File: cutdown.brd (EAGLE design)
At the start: 94 x 100.3 mm, 133 parts, among them J1 RBF_PLUG, Q1 IPB120P04P4L03ATMA1, Q2 SBC817-40LT1G, Q3 SBC817-40LT1G, SW1 M2012LL2W30, U1 ATSAMD21G-A, U2 ATTINY85V-10S, U3 MPL3115A2, U4 R-783.3-0.5_DC-DC, U5 R-783.3-0.5_DC-DC, U6 CD4013B, U7 MC14106BDR2G, X1 ZX62D-B-5PA8, X2 BU-SMA-V, X3 JST-XH-02-PIN-LONG-PAD, X4 JST-XH-02-PIN-LONG-PAD

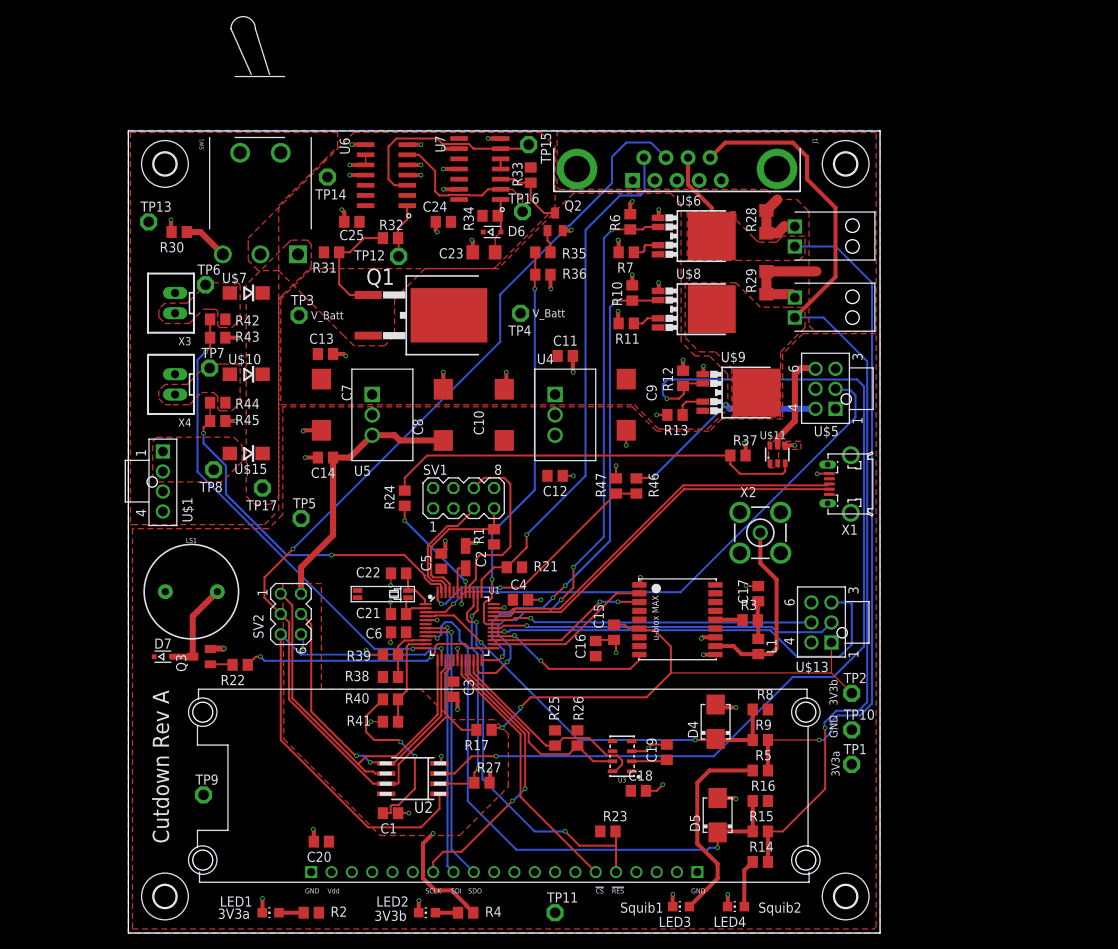
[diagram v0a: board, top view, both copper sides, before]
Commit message: Rev B Hardware
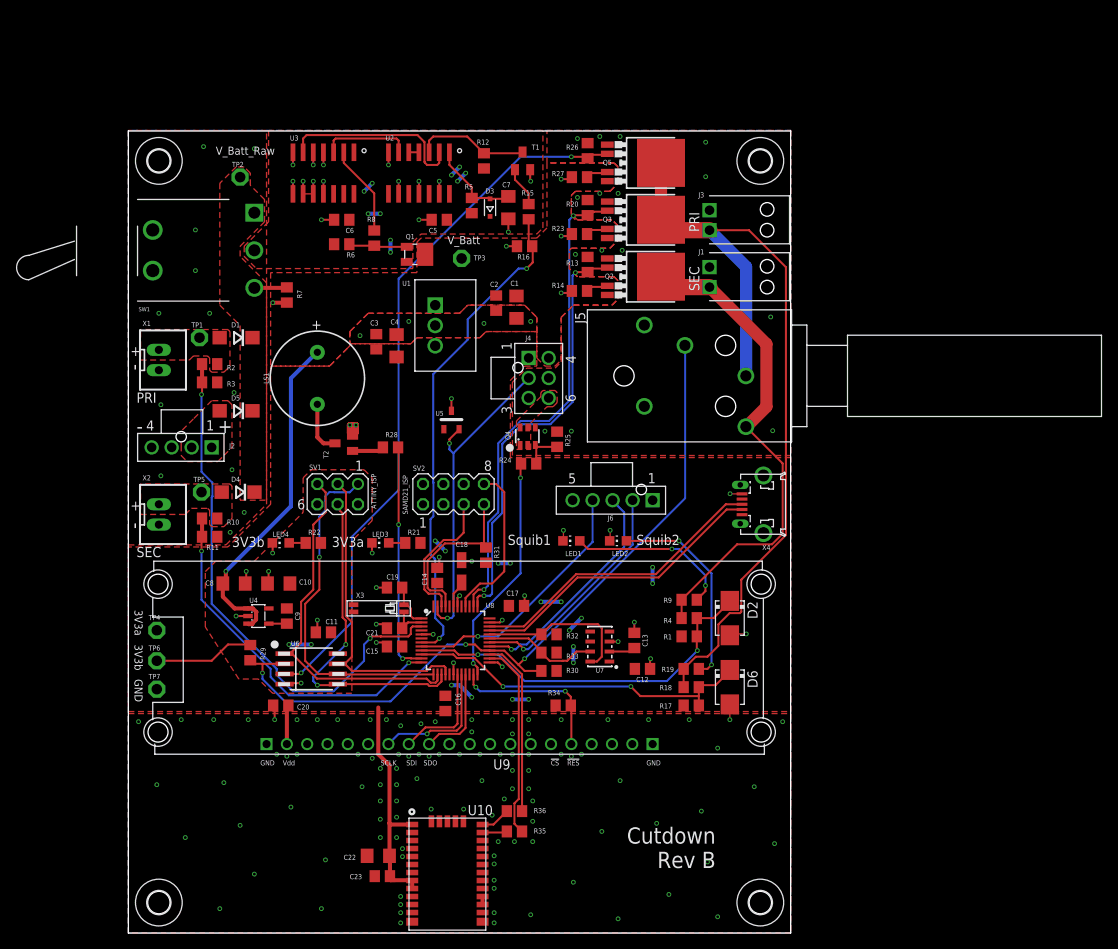
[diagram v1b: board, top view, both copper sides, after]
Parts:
- removed C24, C25: 100n, resistor:C0805
- removed D7: 1N4148, diode:SOD323-R
- removed L1: 27n, rcl:L0805
- removed R37, R38, R39, R40, R41, R43, R45, R47: 10.0K, resistor:R0805
- removed R42, R44, R46: 80.6k, rcl:R0805
- removed TP10, TP11, TP12, TP13, TP14, TP15, TP16, TP17, TP8, TP9: TPSPAD1-13, testpad:P1-13
- removed U$1: 1053091304, Dector_Parts_TR:1053091304
- removed U$10, U$15, U$7: CDBA340L-G, Dector_Parts_TR:DO214AC
- removed U$11: RTQ020N03, Dector_Parts_TR:SC-95(TSMT6)
- removed U$12: NHD-0216CW-AW3, Dector_Parts_TR:NHD-0216CW-AW3
- removed U$13, U$5: 1053101206, Dector_Parts_TR:1053101206
- removed U$14: MC-146-32.7680KA-A0, Dector_Parts_TR:MC-146
- removed U$2, U$3: DECTOR_PARTS_TR_NANOFIT_1X2_RA, Solar Cell Carrier Board:DECTOR_PARTS_TR_NANOFIT_1X2_RIGHTANGLE
- removed U$4: MAX-M8, ubloxLib:MAX-M8
- removed U$6, U$8, U$9: BTS500600-1TEA, Dector_Parts_TR:PG-TO252-5-11
- added D1: CDBA340L-G, Dector_Parts_TR:DO214AC
- added D2: 1SMB5913BT3G, 1smb59xx_10:DO214AA
- added D3: 1N4148, diode:SOD323-R
- added J2: 1053091304, Dector_Parts_TR:1053091304
- added J3: DECTOR_PARTS_TR_NANOFIT_1X2_RA, Solar Cell Carrier Board:DECTOR_PARTS_TR_NANOFIT_1X2_RIGHTANGLE
- added J4: 1053101206, Dector_Parts_TR:1053101206
- added J5: RN114BPC, Dector_Parts_TR:RN114BPC
- added J6: 1053091305, Dector_Parts_TR:1053091305
- added Q4: RTQ020N03, Dector_Parts_TR:SC-95(TSMT6)
- added Q5: BTS50060-1TEA, Dector_Parts_TR:PG-TO252-5-11
- added R18, R20: 10.0K, resistor:R0805
- added R19: 820, rcl:R0805
- added T1, T2: SBC817-40LT1G, transistor-neu-to92:SOT23
- added U10: CAM-M8C-0, Dector_Parts_TR:CAM_M8C
- added U8: ATSAMD21G-A, samd21_lib:TQFP-48
- added U9: NHD-0216CW-AW3, Dector_Parts_TR:NHD-0216CW-AW3
- C1, C4: value 100n -> 10u; device resistor:C0805 -> rcl:C1206
- C10, C7: device rcl:CT7343 -> rcl:C1206
- C17: value 10n -> 100n; device rcl:C0805 -> resistor:C0805
- C18: value 100n -> 1u; device resistor:C0805 -> rcl:CT3216
- C19: value 100n -> 22p; device resistor:C0805 -> rcl:C0805
- C2: value 1u -> 100n; device rcl:CT3216 -> resistor:C0805
- C22: value 22p -> 10u; device rcl:C0805 -> rcl:C1206
- C23: value 10u -> 100n; device rcl:C1206 -> resistor:C0805
- C8: value 10u -> 1u; device rcl:CT7343 -> rcl:C1206
- C9: value 10u -> 10n; device rcl:CT7343 -> rcl:C0805
- D4, D5: value 1SMB5913BT3G -> CDBA340L-G; device 1smb59xx_10:DO214AA -> Dector_Parts_TR:DO214AC
- D6: value 1N4148 -> 1SMB5913BT3G; device diode:SOD323-R -> 1smb59xx_10:DO214AA
- J1: value RBF_PLUG -> DECTOR_PARTS_TR_NANOFIT_1X2_RA; device SparkFun-Connectors:DB9 -> Solar Cell Carrier Board:DECTOR_PARTS_TR_NANOFIT_1X2_RIGHTANGLE
- Q1: value IPB120P04P4L03ATMA1 -> SI2347DS-T1-GE3; device Dector_Parts_TR:TO263-3-2 -> Dector_Parts_TR:SI1247DS
- Q2, Q3: value SBC817-40LT1G -> BTS50060-1TEA; device transistor-neu-to92:SOT23 -> Dector_Parts_TR:PG-TO252-5-11
- R1, R11, R13, R25, R26: value 1k -> 10.0K; device rcl:R0805 -> resistor:R0805
- R10: value 10.0K -> 80.6k; device resistor:R0805 -> rcl:R0805
- R14: value 820 -> 1k
- R15: value 10.0K -> 2.00K
- R2: value 130 -> 80.6k
- R21: value 10.0K -> 130; device resistor:R0805 -> rcl:R0805
- R22: value 180 -> 130
- R23, R27, R31, R32, R33: value 10.0K -> 1k; device resistor:R0805 -> rcl:R0805
- R24: value 100 -> 130
- R28: value 0 -> 2.00K; device rcl:R1206 -> resistor:R0805
- R29: value 0 -> 10.0K; device rcl:R1206 -> resistor:R0805
- R3: value 10 -> 10.0K; device rcl:R0805 -> resistor:R0805
- R30: value 10.0 -> 10.0K
- R34: value 49.9K -> 10.0K
- R35: value 2.00K -> 220; device resistor:R0805 -> rcl:R0805
- R36: value 10.0K -> 220; device resistor:R0805 -> rcl:R0805
- R4: value 130 -> 10.0K; device rcl:R0805 -> resistor:R0805
- R5: value 820 -> 49.9K; device rcl:R0805 -> resistor:R0805
- R7: value 1k -> 10.0; device rcl:R0805 -> resistor:R0805
- R9: value 10.0K -> 820; device resistor:R0805 -> rcl:R0805
- SV1: value SAMD21_ISP -> ATTINY_ISP; device con-lstb:MA04-2 -> con-lstb:MA03-2
- SV2: value ATTINY_ISP -> SAMD21_ISP; device con-lstb:MA03-2 -> con-lstb:MA04-2
- U1: value ATSAMD21G-A -> R-783.3-0.5_DC-DC; device samd21_lib:TQFP-48 -> Dector_Parts_TR:R-783P3-0P5_DC-DC
- U2: value ATTINY85V-10S -> MC14106BDR2G; device _hhn_attiny25_45_85:SOIC8_EIAJ_208MIL -> Dector_Parts_TR:SOIC-14
- U3: value MPL3115A2 -> CD4013B; device SparkFun-Sensors:LGA-8-5X3 -> Dector_Parts_TR:SOIC-14
- U4: value R-783.3-0.5_DC-DC -> LT1761IS5-3.3; device Dector_Parts_TR:R-783P3-0P5_DC-DC -> Dector_Parts_TR:TSOT23-5
- U5: value R-783.3-0.5_DC-DC -> MCP9700T-E/TT; device Dector_Parts_TR:R-783P3-0P5_DC-DC -> Dector_Parts_TR:MCP9700T-E/TT
- U6: value CD4013B -> ATTINY85V-10S; device Dector_Parts_TR:SOIC-14 -> _hhn_attiny25_45_85:SOIC8_EIAJ_208MIL
- U7: value MC14106BDR2G -> MPL3115A2; device Dector_Parts_TR:SOIC-14 -> SparkFun-Sensors:LGA-8-5X3
- X1: value ZX62D-B-5PA8 -> JST-XH-02-PIN-LONG-PAD; device zx62d-b-5pa8-oshpark_10:ZX62D-B-5PA8 -> Rembrandt Electronics - JST XH Connectors v1-0:JST-XH-02-PACKAGE-LONG-PAD
- X2: value BU-SMA-V -> JST-XH-02-PIN-LONG-PAD; device con-coax:BU-SMA-V -> Rembrandt Electronics - JST XH Connectors v1-0:JST-XH-02-PACKAGE-LONG-PAD
- X3: value JST-XH-02-PIN-LONG-PAD -> MC-146-32.7680KA-A0; device Rembrandt Electronics - JST XH Connectors v1-0:JST-XH-02-PACKAGE-LONG-PAD -> Dector_Parts_TR:MC-146
- X4: value JST-XH-02-PIN-LONG-PAD -> ZX62D-B-5PA8; device Rembrandt Electronics - JST XH Connectors v1-0:JST-XH-02-PACKAGE-LONG-PAD -> zx62d-b-5pa8-oshpark_10:ZX62D-B-5PA8
- moved TP2 100.0 mm to (14.0, 94.5)
- moved TP1 97.4 mm to (8.89, 74.4)
- moved X1 90.0 mm to (3.81, 71.6), turned to 270 degrees
- moved R15 82.7 mm to (50.0, 90.2), turned to 270 degrees
- moved U3 81.9 mm to (24.4, 95.0)
- moved R29 79.4 mm to (15.2, 35.1), turned to 270 degrees
- moved R5 79.3 mm to (42.9, 90.9), turned to 90 degrees
- moved C23 79.0 mm to (31.8, 7.11)
- moved D5 78.6 mm to (13.5, 65.3), turned to 180 degrees
- moved Q3 78.3 mm to (65.3, 89.2), turned to 270 degrees
- moved X4 77.2 mm to (81.5, 53.6), turned to 180 degrees
- moved R27 76.7 mm to (56.4, 94.5)
- moved R8 76.2 mm to (30.7, 86.9), turned to 270 degrees
- moved U2 75.7 mm to (36.3, 95.0), turned to 180 degrees
- moved R16 75.3 mm to (49.5, 85.9)
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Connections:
- removed net !GPS_RESET!: U$4.9_RESET_N, U1.28
- removed net !OLED_CS!: U$12.P$15, U1.19
- removed net !SAMD21_ARM!: J1.6, R21.2, U1.37
- removed net 3V3A_VMON: R38.2, R39.1, U1.10
- removed net 3V3B_VMON: R40.2, R41.1, U1.11
- removed net ATTINY_SCK/!ATTINY_ARM!: J1.7, R17.2, SV2.3, U1.16, U2.7
- removed net BATT1_VMON: R42.1, R43.1, U1.12
- removed net BATT2_VMON: R44.1, R45.1, U1.47
- removed net GPS_ANTENNA: L1.1, U$4.11_RF_IN, X2.1
- removed net N$25: C21.2, U$14.P$4, U1.2
- removed net N$7: R42.2, TP6.TP, U$7.A, X3.1
- removed net RADIO_GPIO2: U$13.5, U1.32
- removed net SQUIB1: J1.8, R5.2, R9.2, U$2.P$1, U$6.TAB
- removed net SQUIB1_GATE: R6.1, U$6.2, U1.23
- removed net SQUIB1_VMON: D4.C, R8.2, R9.1, U1.4
- removed net SQUIB2: J1.9, R14.2, R15.2, U$3.P$1, U$8.TAB, U$9.TAB
- removed net SQUIB2_GATE: R10.1, U$8.2, U1.24
- removed net SQUIB2_GATE_BCKP: R12.1, U$9.2, U2.3
- removed net SQUIB2_VMON: D5.C, R15.1, R16.2, U1.9
- removed net SQUIB_FIRED: R27.1, U1.38, U2.2
- removed net VBATT_VMON: R46.2, R47.2, U1.48
- new net !SYSTEM_ARM!: J5.TS, R29.2, R30.2, U6.2, U8.28
- new net AREF: U8.4
- new net ATN: U8.22
- new net ATTINY_SCK: SV1.3, U6.7, U8.16
- new net ATTINY_SQUIB_PRI: Q5.2, R26.1, U6.3
- new net BATTPRI: D1.A, R2.2, TP1.TP, X1.1
- new net BATTPRI_VMON: R2.1, R3.1, U8.3
- new net BATTSEC: D4.A, R10.2, TP5.TP, X2.1
- new net BATTSEC_VMON: R10.1, R11.1, U8.12
- new net N$27: C9.2, U4.4
- new net N$28: R36.1, U10.26
- new net RX_LED: U8.48
- new net SAMD21_SQUIB_BCKP: Q2.2, R13.1, U8.37
- new net SAMD21_SQUIB_PRI: Q3.2, R20.1, U8.38
- new net SPARE_GPIO1: J6.4, U8.8
- new net SPARE_GPIO2: U8.25
- new net SQUIB_BCKP: J1.P$1, J5.R, Q2.TAB, R4.2, R9.2
- new net SQUIB_BCKP_VMON: D2.C, R1.2, R4.1, U8.9
- new net SQUIB_PRI: J3.P$1, J5.S, Q3.TAB, Q5.TAB, R18.2, R19.2
- new net SQUIB_PRI_VMON: D6.C, R17.2, R18.1, U8.10
- new net TX_LED: U8.39
- new net USB_HOST_EN: U8.41
- net !ATTINY_RST!: now also SV1.5, U6.1, U8.14; no longer SV2.5, U1.14, U2.1
- net !OLED_RES!: now also R34.2, U8.23, U9.P$16; no longer R23.2, U$12.P$16, U1.39
- net !SAMD21_RST!: now also SV2.8, U8.40; no longer SV1.6, U1.40
- net 1.2V: now also C18.+, U8.43; no longer C2.+, U1.43
- net ATTINY_MISO_DO: now also SV1.1, U6.6, U8.13; no longer SV2.1, U1.13, U2.6
- net ATTINY_MOSI_DI: now also SV1.4, U6.5, U8.15; no longer SV2.4, U1.15, U2.5
- net BUZZER: now also R28.2, U8.11; no longer R22.1, U1.25
- net CLK: now also U2.6, U3.3; no longer TP15.TP, U6.3, U7.6
- net GND: now also C10.2, C18.-, C19.1, C2.2, C22.2, C7.2, C8.2, D2.A, D6.A, J1.P$2, J2.3, J2.4, J3.P$2, J4.3, J4.5, J5.T, J6.5, Q2.1, Q3.1, Q4.4, Q5.1, R11.2, R13.2, R14.1, R16.2, R20.2, R23.1, R25.2, R26.2, R27.1, R3.2, R7.2, SV1.6, SV2.1, SV2.2, SV2.3, SV2.4, T1.2, T2.2, TP7.TP, U1.2, U10.10, U10.11, U10.12, U10.13, U10.14, U10.15, U10.18, U10.19, U10.21, U10.22, U10.27, U10.31, U10.4, U10.5, U2.11, U2.13, U2.7, U2.9, U3.10, U3.11, U3.4, U3.5, U3.7, U3.8, U3.9, U5.P$3, U7.3, U8.18, U8.35, U8.42, U8.5, U9.P$1, U9.P$10, U9.P$11, U9.P$12, U9.P$13, U9.P$14, U9.P$15, U9.P$17, U9.P$18, U9.P$19, U9.P$20, U9.P$3, U9.P$4, U9.P$5, U9.P$6, X1.2, X4.5; no longer C10.-, C18.2, C19.2, C2.-, C22.1, C24.2, C25.2, C7.-, C8.-, C9.-, D4.A, D5.A, J1.1, J1.2, J1.3, J1.4, J1.5, Q2.2, Q3.2, R10.2, R11.1, R12.2, R13.1, R27.2, R28.1, R28.2, R29.1, R29.2, R30.2, R36.2, R37.2, R39.2, R41.2, R43.2, R45.2, R47.1, R6.2, R7.1, SV1.1, SV1.2, SV1.3, SV1.4, SV2.6, TP10.TP, TP11.TP, TP13.TP, TP5.TP, TP9.TP, U$1.3, U$1.4, U$11.4, U$12.P$1, U$12.P$10, U$12.P$11, U$12.P$12, U$12.P$13, U$12.P$14, U$12.P$17, U$12.P$18, U$12.P$19, U$12.P$20, U$12.P$3, U$12.P$4, U$12.P$5, U$12.P$6, U$13.6, U$2.P$2, U$3.P$2, U$4.10_GND, U$4.12_GND, U$4.1_GND, U$5.3, U$5.5, U$6.1, U$8.1, U$9.1, U1.18, U1.35, U1.42, U1.5, U2.4, U3.3, U5.2, U6.10, U6.11, U6.5, U6.7, U6.8, U6.9, U7.11, U7.13, U7.7, U7.9, X1.5, X2.3, X2.4, X2.5, X3.2, X4.2
- net GPS_RX: now also R36.2, U8.27; no longer U$4.3_RXD, U1.27
- net GPS_TX: now also R35.2, U8.26; no longer U$4.2_TXD, U1.26
- net HEATER_GATE: now also U8.24; no longer U1.41
- net N$1: now also D5.A, J2.1, J2.2; no longer TP8.TP, U$1.1, U$1.2, U$15.A
- net N$10: now also U10.16, U10.17; no longer C17.1, L1.2, R3.1
- net N$11: now also R35.1, U10.25; no longer R3.2, U$4.14_VCC_RF
- net N$12: now also C21.2, U8.2, X3.P$4; no longer R44.2, TP7.TP, U$10.A, X4.1
- net N$13: now also LED3.A, R21.1; no longer LED1.A, R2.1
- net N$14: now also Q2.4, R14.2; no longer R7.2, U$6.4
- net N$15: now also LED4.A, R22.1; no longer LED2.A, R4.1
- net N$16: now also LED1.A, R9.1; no longer LED3.A, R5.1
- net N$17: now also R8.1, U3.2; no longer R32.1, TP12.TP, U6.1
- net N$18: now also U2.4, U2.5; no longer U7.4, U7.5
- net N$19: now also Q3.4, R23.2; no longer R11.2, U$8.4
- net N$2: now also R28.1, T2.1; no longer Q3.1, R22.2
- net N$20: now also Q5.4, R27.2; no longer R13.2, U$9.4
- net N$21: now also LED2.A, R19.1; no longer LED4.A, R14.1
- net N$22: now also J4.6, Q4.1, Q4.2, Q4.5, Q4.6; no longer U$11.1, U$11.2, U$11.5, U$11.6, U$5.6
- net N$23: now also Q4.3, R25.1; no longer R37.1, U$11.3
- net N$24: now also C19.2, U8.1, X3.P$1; no longer C22.2, U$14.P$1, U1.1
- net N$26: now also LS1.-, T2.3; no longer D7.A, LS1.+, Q3.3
- net N$3: now also R7.1; no longer R30.1
- net N$4: now also Q1.G, R6.2, R8.2; no longer Q1.1, R31.2, R32.2
- net N$5: now also C7.1, D3.A, R5.2, U2.1; no longer C23.1, D6.A, R34.2, U7.1
- net N$6: now also R15.1, T1.1; no longer Q2.1, R35.1
- net N$8: now also R12.2, T1.3, U2.3; no longer Q2.3, R33.2, U7.3
- net N$9: now also C13.1, U7.2; no longer C19.1, U3.2
- net OLED_MISO: now also U8.21, U9.P$9; no longer U$12.P$9, U1.8
- net OLED_MOSI: now also U8.19, U9.P$8; no longer U$12.P$8, U1.7
- net OLED_SCLK: now also U8.20, U9.P$7; no longer U$12.P$7, U1.20
- net PRESSURE_SCL: now also R32.1, U7.8, U8.32; no longer R25.1, U1.22, U3.8
- net PRESSURE_SDA: now also R33.1, U7.7, U8.31; no longer R26.1, U1.21, U3.7
- net PWR_OFF: now also R15.2, R16.1, U8.7; no longer R35.2, R36.1, U1.31
- net RADIO_RX: now also J6.3, U8.29; no longer U$13.3, U1.29
- net RADIO_TX: now also J6.2, U8.30; no longer U$13.2, U1.30
- net SAMD21_SWCLK: now also R31.1, SV2.7, U8.45; no longer R1.1, SV1.7, U1.45
- net SAMD21_SWDIO: now also SV2.5, U8.46; no longer SV1.5, U1.46
- net SET: now also U2.2, U3.6; no longer TP16.TP, U6.6, U7.2
- net THERMISTOR_VOUT: now also J4.2, U5.P$2, U8.47; no longer U$5.2, U1.3
- net USB_D+: now also U8.34, X4.3; no longer U1.34, X1.3
- net USB_D-: now also U8.33, X4.2; no longer U1.33, X1.2
- net VBATT_RAW: now also D1.C, D4.C, D5.C, TP2.TP; no longer TP17.TP, U$10.C, U$15.C, U$7.C
- net VCC_1: now also C14.1, C15.1, C17.1, C22.1, C23.1, J4.1, J6.1, R1.1, R17.1, R21.2, R30.1, R31.2, R32.2, R33.2, R34.1, SV2.6, TP4.TP, U1.3, U10.1, U10.8, U10.9, U5.P$1, U7.1, U7.4, U8.17, U8.36, U8.44, U8.6, U9.P$2; no longer C10.+, C18.1, C5.1, C6.1, D7.C, LS1.-, R1.2, R16.1, R2.2, R21.1, R23.1, R25.2, R26.2, R38.1, R8.1, SV1.8, TP1.TP, U$12.P$2, U$4.7_VCC_IO, U$4.8_VCC, U$5.1, U1.17, U1.36, U1.44, U1.6, U3.1, U3.4, U4.3
- net VCC_2: now also C10.1, C11.1, C9.1, R22.2, R29.1, SV1.2, TP6.TP, U4.5, U6.8; no longer C1.1, C14.1, C15.1, C8.+, R17.1, R4.2, R40.1, SV2.2, TP2.TP, U$13.1, U$4.6_V_BCKP, U2.8, U5.3
- net VSW: now also C5.1, C6.1, D3.C, Q1.S, R12.1, R5.1, R6.1, U2.14, U3.14; no longer C24.1, C25.1, D6.C, Q1.3, R31.1, R33.1, R34.1, TP14.TP, U6.14, U7.14
- net V_BATT: now also C1.1, C2.1, C8.1, J4.4, LS1.+, Q1.D, Q2.5, Q3.5, Q5.5, U1.1, U4.3; no longer C11.1, C13.1, C7.+, C9.+, Q1.2, R46.1, TP4.TP, U$5.4, U$6.5, U$8.5, U$9.5, U5.1
- net V_USB: now also X4.1; no longer X1.1
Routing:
- net ATTINY_SCK/!ATTINY_ARM!: track 136.1 -> 0.00 mm, vias 1 -> 0
- net SQUIB2_GATE_BCKP: track 126.0 -> 0.00 mm, vias 2 -> 0
- net VCC_2: track 134.8 -> 15.3 mm, vias 5 -> 2
- net SQUIB2: track 119.1 -> 0.00 mm, vias 1 -> 0
- net SQUIB_PRI: track 0.00 -> 104.7 mm
- net !SYSTEM_ARM!: track 0.00 -> 95.3 mm, vias 0 -> 3
- net SQUIB1: track 94.6 -> 0.00 mm, vias 1 -> 0
- net ATTINY_SQUIB_PRI: track 0.00 -> 89.2 mm, vias 0 -> 2
- net SQUIB1_GATE: track 75.0 -> 0.00 mm, vias 4 -> 0
- net SQUIB2_VMON: track 72.0 -> 0.00 mm, vias 2 -> 0
- net GND: track 144.4 -> 77.3 mm, vias 71 -> 181
- net BATTPRI_VMON: track 0.00 -> 66.8 mm, vias 0 -> 2
- net !SAMD21_ARM!: track 65.2 -> 0.00 mm, vias 1 -> 0
- net SQUIB2_GATE: track 62.4 -> 0.00 mm, vias 4 -> 0
- net SQUIB_BCKP: track 0.00 -> 61.7 mm
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- added copper zone on layer 1, net BATTPRI
- added copper zone on layer 1, net BATTSEC
- removed copper zone on layer 1, net N$12
- removed copper zone on layer 1, net N$7
- removed copper zone on layer 1, net SQUIB1
- removed copper zone on layer 1, net SQUIB2
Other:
- board size 94 x 100.3 mm -> 82.8 x 100.3 mm
- board text added: "+"
- board text added: "-"
- board text added: "Cutdown Rev B"
- board text added: "PRI"
- board text added: "SEC"
- board text added: "V_Batt_Raw"
- board text removed: "Cutdown Rev A"
